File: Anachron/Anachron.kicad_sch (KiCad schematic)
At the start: 0 parts

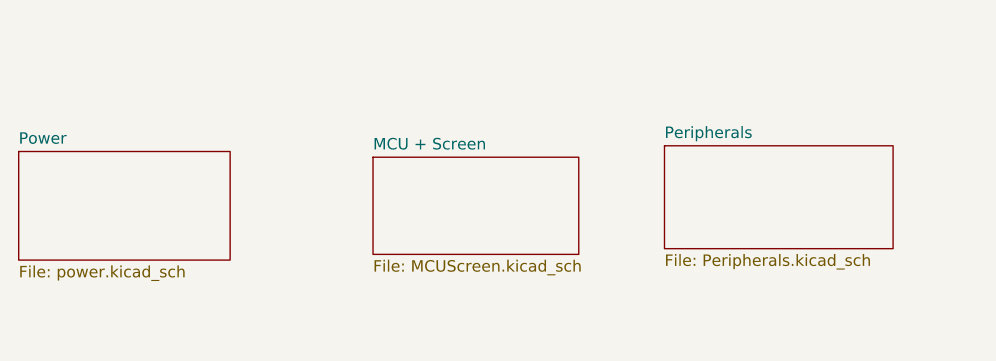
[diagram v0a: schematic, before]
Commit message: layed everything outttt
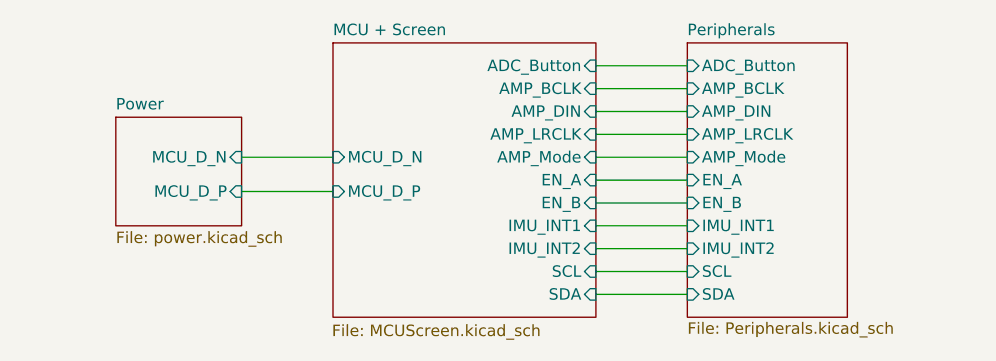
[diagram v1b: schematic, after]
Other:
- sheet MCU + Screen ports: added ADC_Button, AMP_BCLK, AMP_DIN, AMP_LRCLK, AMP_Mode, EN_A, EN_B, IMU_INT1, IMU_INT2, MCU_D_N, MCU_D_P, SCL, SDA; removed none
- sheet Peripherals ports: added ADC_Button, AMP_BCLK, AMP_DIN, AMP_LRCLK, AMP_Mode, EN_A, EN_B, IMU_INT1, IMU_INT2, SCL, SDA; removed none
- sheet Power ports: added MCU_D_N, MCU_D_P; removed none

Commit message: layout power
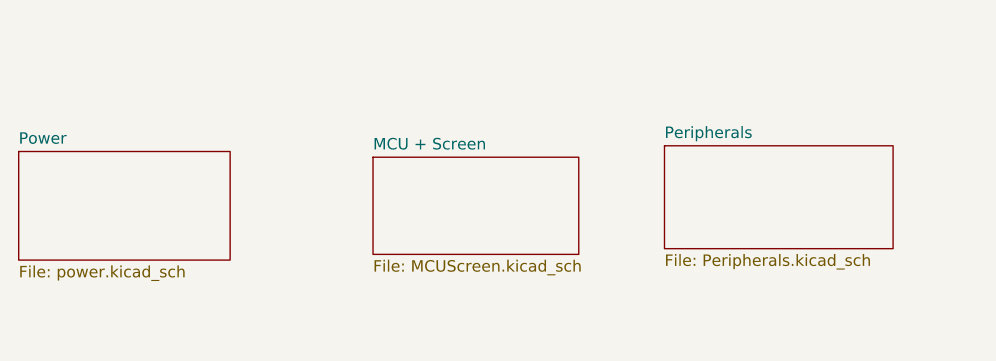
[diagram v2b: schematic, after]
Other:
- sheet MCU + Screen ports: added none; removed ADC_Button, AMP_BCLK, AMP_DIN, AMP_LRCLK, AMP_Mode, EN_A, EN_B, IMU_INT1, IMU_INT2, MCU_D_N, MCU_D_P, SCL, SDA
- sheet Peripherals ports: added none; removed ADC_Button, AMP_BCLK, AMP_DIN, AMP_LRCLK, AMP_Mode, EN_A, EN_B, IMU_INT1, IMU_INT2, SCL, SDA
- sheet Power ports: added none; removed MCU_D_N, MCU_D_P
